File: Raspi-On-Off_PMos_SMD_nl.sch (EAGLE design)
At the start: 32 parts, among them IC1 74AUC1G17, T1 FDC6327C, T2 FDC6327C, T3 BSS123, T4 IRF7416, T5 IRLML0030, X1 MKDSN1,5/2-5,08

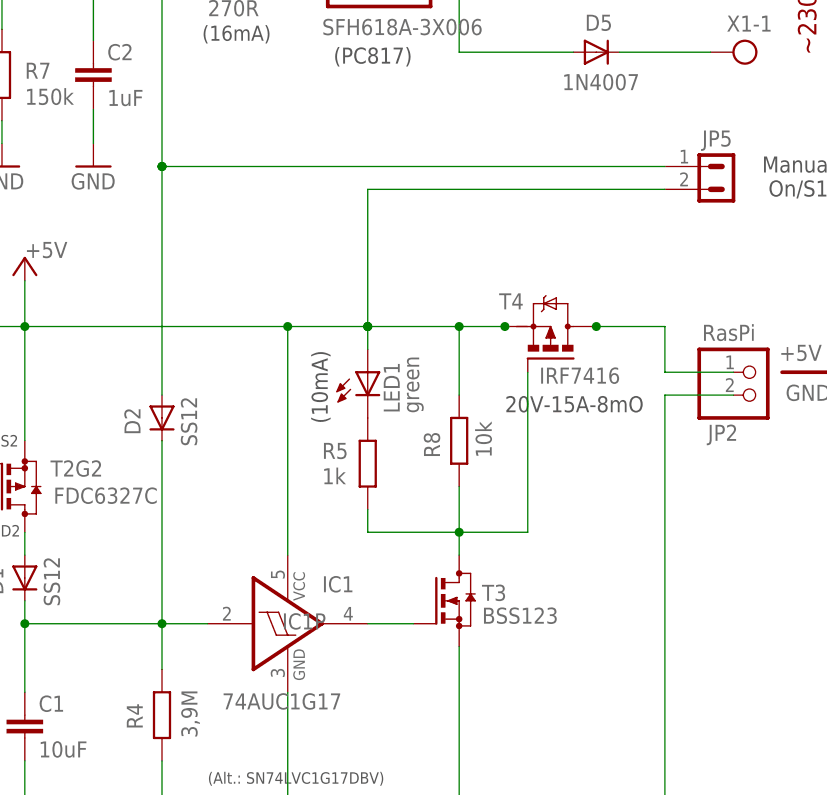
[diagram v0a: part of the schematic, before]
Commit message: Add files via upload
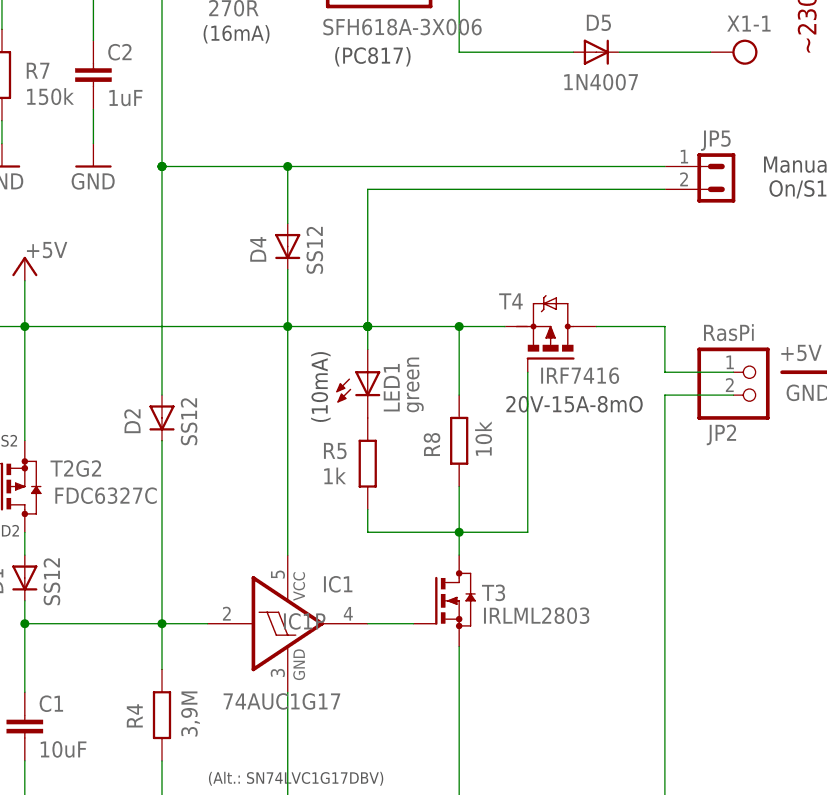
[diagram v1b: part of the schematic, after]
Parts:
- added D4: SS12, diode2:MBR0520LT
- T3: value BSS123 -> IRLML2803
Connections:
- net +5V: now also D4.C
- net N$8: now also D4.A
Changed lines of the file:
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@@
 <part name="GND5" library="supply1" deviceset="GND" device=""/>
 <part name="R3" library="rcl" deviceset="R-EU_" device="R0805" value="270R"/>
-<part name="T3" library="transistor-small-signal" deviceset="BSS123" device="23" value="BSS123"/>
+<part name="T3" library="transistor-small-signal" deviceset="BSS123" device="23" value="IRLML2803"/>
 <part name="LED2" library="led" deviceset="LED" device="3MM" value="red"/>
 <part name="T5" library="transistor-small-signal" deviceset="BSS123" device="23" value="IRLML0030"/>
@@
 <part name="JP6" library="con-lstc" deviceset="MA02-1" device="1" value="Relais"/>
 <part name="D3" library="diode2" deviceset="MBR0520LT" device="" value="SS12"/>
+<part name="D4" library="diode2" deviceset="MBR0520LT" device="" value="SS12"/>
 </parts>
 <sheets>
@@
 <attribute name="VALUE" x="55.88" y="49.7586" size="1.778" layer="96"/>
 </instance>
+<instance part="D4" gate="G$1" x="138.43" y="87.63" smashed="yes" rot="R270">
+<attribute name="NAME" x="136.0424" y="85.725" size="1.778" layer="95" rot="R90"/>
+<attribute name="VALUE" x="142.3289" y="84.455" size="1.778" layer="96" rot="R90"/>
+</instance>
 </instances>
 <busses>
@@
 <pinref part="T4" gate="G$1" pin="S"/>
 <pinref part="T4" gate="G$1" pin="S@1"/>
-<junction x="162.56" y="78.74"/>
 <pinref part="T4" gate="G$1" pin="S@2"/>
 <pinref part="IC1" gate="P" pin="VCC"/>
@@
 <pinref part="D3" gate="G$1" pin="C"/>
 <junction x="60.96" y="53.34"/>
+<pinref part="D4" gate="G$1" pin="C"/>
+<wire x1="138.43" y1="78.74" x2="138.43" y2="85.09" width="0.1524" layer="91"/>
 </segment>
 <segment>
@@
 <pinref part="T4" gate="G$1" pin="D"/>
 <pinref part="T4" gate="G$1" pin="D@1"/>
-<junction x="172.72" y="78.74"/>
 <pinref part="T4" gate="G$1" pin="D@2"/>
 <pinref part="T4" gate="G$1" pin="D@3"/>
@@
 <wire x1="124.46" y1="71.12" x2="124.46" y2="96.52" width="0.1524" layer="91"/>
 <pinref part="JP5" gate="G$1" pin="1"/>
-<wire x1="124.46" y1="96.52" x2="180.34" y2="96.52" width="0.1524" layer="91"/>
+<wire x1="124.46" y1="96.52" x2="138.43" y2="96.52" width="0.1524" layer="91"/>
 <junction x="124.46" y="96.52"/>
+<wire x1="138.43" y1="96.52" x2="180.34" y2="96.52" width="0.1524" layer="91"/>
 <wire x1="124.46" y1="96.52" x2="124.46" y2="116.84" width="0.1524" layer="91"/>
 <junction x="124.46" y="96.52"/>
@@
 <junction x="99.06" y="116.84"/>
 <wire x1="81.28" y1="116.84" x2="99.06" y2="116.84" width="0.1524" layer="91"/>
-</segment>
-</net>
+<pinref part="D4" gate="G$1" pin="A"/>
+<wire x1="138.43" y1="90.17" x2="138.43" y2="96.52" width="0.1524" layer="91"/>
+<junction x="138.43" y="96.52"/>
+</segment>
+</net>

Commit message: Add files via upload
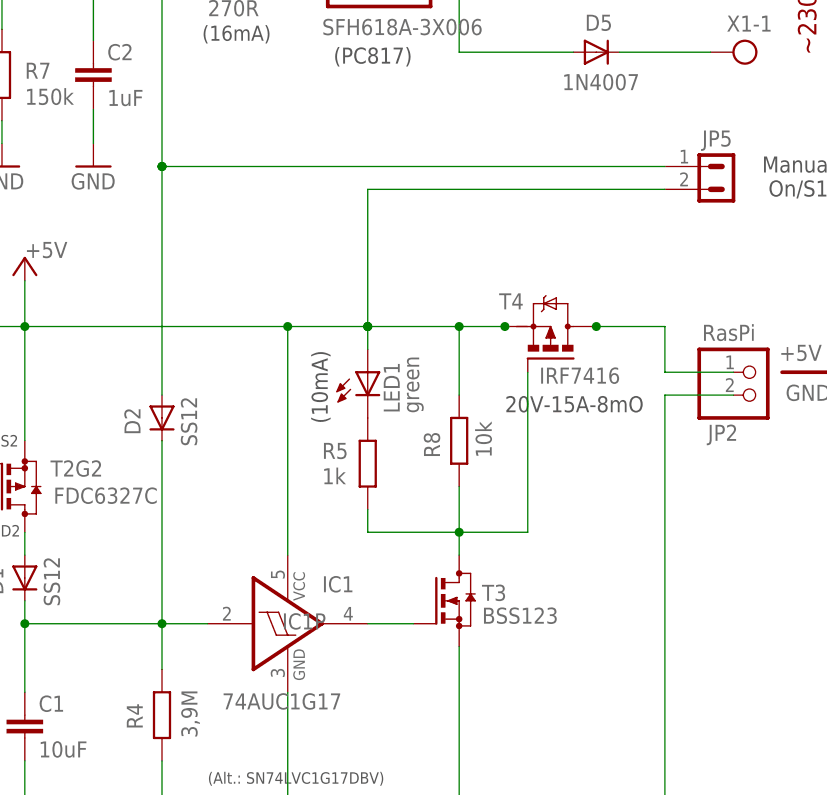
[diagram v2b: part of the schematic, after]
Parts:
- removed D4: SS12, diode2:MBR0520LT
- T3: value IRLML2803 -> BSS123
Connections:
- net +5V: no longer D4.C
- net N$8: no longer D4.A
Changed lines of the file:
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@@
 <part name="GND5" library="supply1" deviceset="GND" device=""/>
 <part name="R3" library="rcl" deviceset="R-EU_" device="R0805" value="270R"/>
-<part name="T3" library="transistor-small-signal" deviceset="BSS123" device="23" value="IRLML2803"/>
+<part name="T3" library="transistor-small-signal" deviceset="BSS123" device="23" value="BSS123"/>
 <part name="LED2" library="led" deviceset="LED" device="3MM" value="red"/>
 <part name="T5" library="transistor-small-signal" deviceset="BSS123" device="23" value="IRLML0030"/>
@@
 <part name="JP6" library="con-lstc" deviceset="MA02-1" device="1" value="Relais"/>
 <part name="D3" library="diode2" deviceset="MBR0520LT" device="" value="SS12"/>
-<part name="D4" library="diode2" deviceset="MBR0520LT" device="" value="SS12"/>
 </parts>
 <sheets>
@@
 <attribute name="VALUE" x="55.88" y="49.7586" size="1.778" layer="96"/>
 </instance>
-<instance part="D4" gate="G$1" x="138.43" y="87.63" smashed="yes" rot="R270">
-<attribute name="NAME" x="136.0424" y="85.725" size="1.778" layer="95" rot="R90"/>
-<attribute name="VALUE" x="142.3289" y="84.455" size="1.778" layer="96" rot="R90"/>
-</instance>
 </instances>
 <busses>
@@
 <pinref part="T4" gate="G$1" pin="S"/>
 <pinref part="T4" gate="G$1" pin="S@1"/>
+<junction x="162.56" y="78.74"/>
 <pinref part="T4" gate="G$1" pin="S@2"/>
 <pinref part="IC1" gate="P" pin="VCC"/>
@@
 <pinref part="D3" gate="G$1" pin="C"/>
 <junction x="60.96" y="53.34"/>
-<pinref part="D4" gate="G$1" pin="C"/>
-<wire x1="138.43" y1="78.74" x2="138.43" y2="85.09" width="0.1524" layer="91"/>
 </segment>
 <segment>
@@
 <pinref part="T4" gate="G$1" pin="D"/>
 <pinref part="T4" gate="G$1" pin="D@1"/>
+<junction x="172.72" y="78.74"/>
 <pinref part="T4" gate="G$1" pin="D@2"/>
 <pinref part="T4" gate="G$1" pin="D@3"/>
@@
 <wire x1="124.46" y1="71.12" x2="124.46" y2="96.52" width="0.1524" layer="91"/>
 <pinref part="JP5" gate="G$1" pin="1"/>
-<wire x1="124.46" y1="96.52" x2="138.43" y2="96.52" width="0.1524" layer="91"/>
+<wire x1="124.46" y1="96.52" x2="180.34" y2="96.52" width="0.1524" layer="91"/>
 <junction x="124.46" y="96.52"/>
-<wire x1="138.43" y1="96.52" x2="180.34" y2="96.52" width="0.1524" layer="91"/>
 <wire x1="124.46" y1="96.52" x2="124.46" y2="116.84" width="0.1524" layer="91"/>
 <junction x="124.46" y="96.52"/>
@@
 <junction x="99.06" y="116.84"/>
 <wire x1="81.28" y1="116.84" x2="99.06" y2="116.84" width="0.1524" layer="91"/>
-<pinref part="D4" gate="G$1" pin="A"/>
-<wire x1="138.43" y1="90.17" x2="138.43" y2="96.52" width="0.1524" layer="91"/>
-<junction x="138.43" y="96.52"/>
-</segment>
-</net>
+</segment>
+</net>
